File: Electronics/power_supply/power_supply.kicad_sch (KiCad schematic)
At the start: 83 parts, among them IC1 TLV76033DBZR, IC2 LM5069MMX-2_NOPB, J1 Conn_01x02_Male, J10 9801-0-15-15-23-27-10-0, J12 9801-0-15-15-23-27-10-0, J13 9801-0-15-15-23-27-10-0, J14 9801-0-15-15-23-27-10-0, J2 9801-0-15-15-23-27-10-0, J3 Conn_01x02_Male, J4 821-22-002-10-001101, J5 9801-0-15-15-23-27-10-0, J6 Conn_01x04_Male, J7 Conn_01x02_Male, J8 Conn_01x02_Male, J9 Conn_01x02_Pin, Q1 IPD90N04S4L04ATMA1, Q3 BC857, U1 R-78B5.0-2.0, U2 INA226, U3 INA226

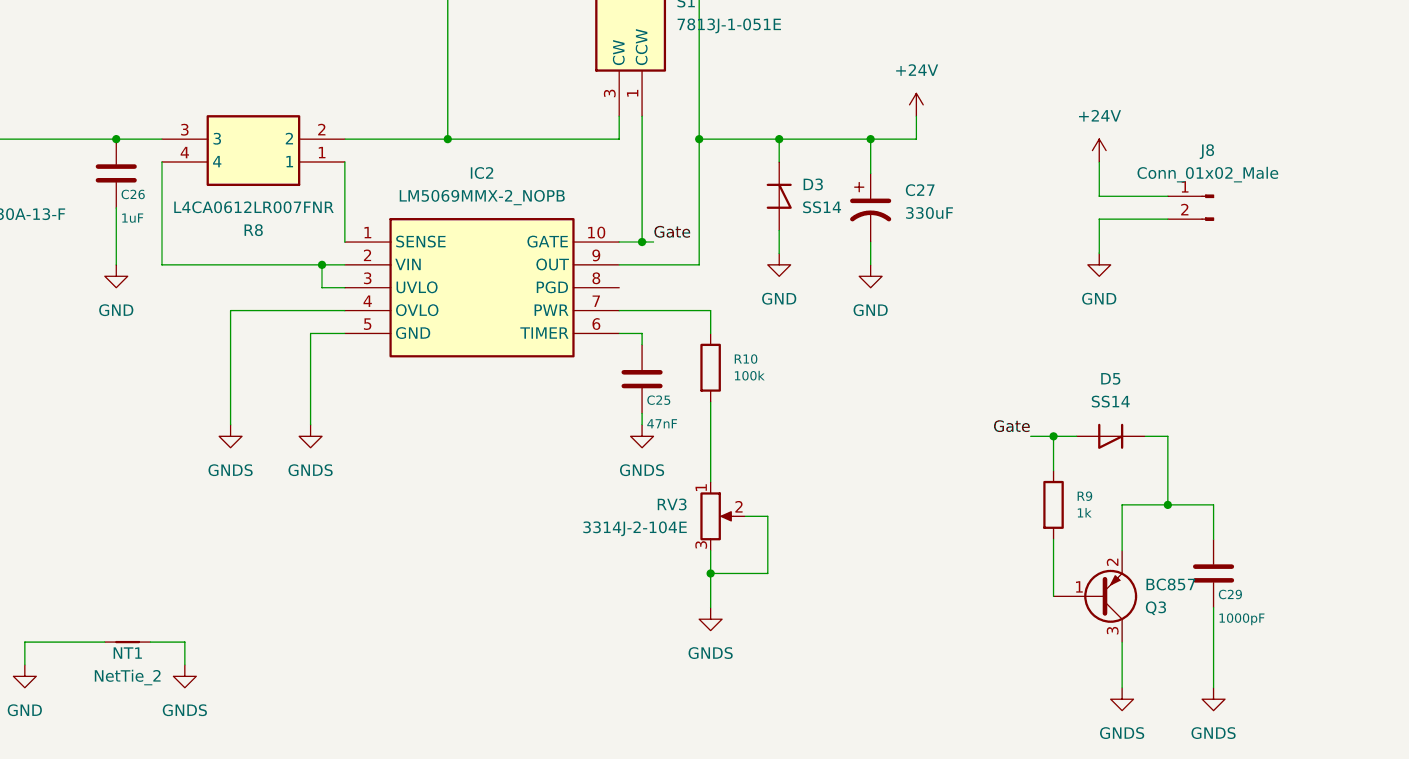
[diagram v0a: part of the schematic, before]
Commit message: PCB fixup
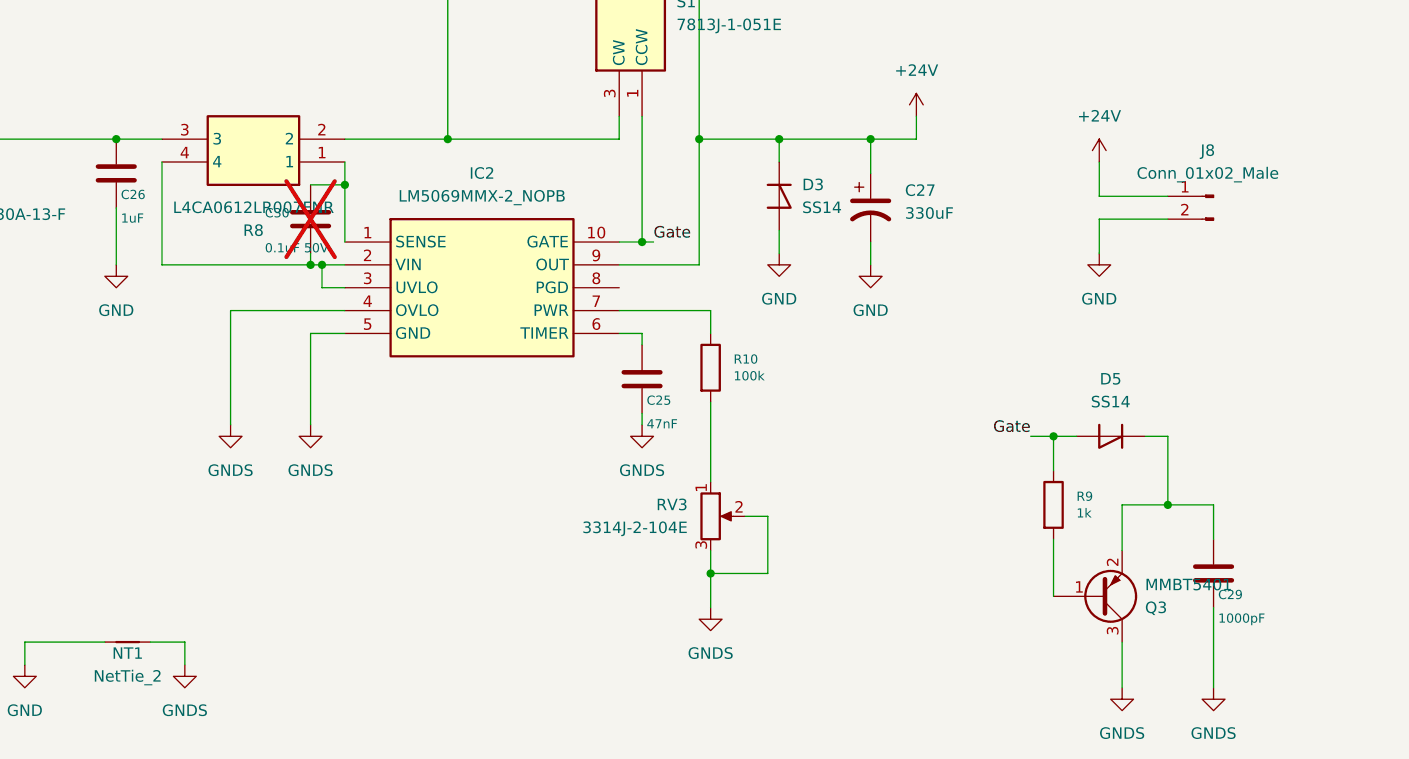
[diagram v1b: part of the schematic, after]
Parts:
- added C30: 0.1uF 50V, Capacitor_SMD:C_0402_1005Metric_Pad0.74x0.62mm_HandSolder, symbol Device:C
- Q3: value BC857 -> MMBT5401; Mouser 583-C857 -> 165-8634
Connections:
- net at IC2.1 (SENSE), R8.1: now also C30.1
- net at IC2.2 (VIN), IC2.3 (UVLO), R8.4: now also C30.2
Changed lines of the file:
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@@
 	)
 	(junction
+		(at 158.75 219.71)
+		(diameter 0)
+		(color 0 0 0 0)
+	)
+	(junction
 		(at 254 246.38)
 		(diameter 0)
@@
 	)
 	(junction
+		(at 162.56 210.82)
+		(diameter 0)
+		(color 0 0 0 0)
+	)
+	(junction
 		(at 351.79 45.72)
 		(diameter 0)
@@
 	(wire
 		(pts
-			(xy 142.24 219.71) (xy 160.02 219.71)
+			(xy 142.24 219.71) (xy 158.75 219.71)
 		)
 		(stroke
@@
 	(wire
 		(pts
-			(xy 162.56 208.28) (xy 162.56 217.17)
+			(xy 162.56 208.28) (xy 162.56 210.82)
 		)
 		(stroke
@@
 	(wire
 		(pts
+			(xy 162.56 210.82) (xy 162.56 217.17)
+		)
+		(stroke
+			(width 0)
+			(type default)
+		)
+	)
+	(wire
+		(pts
 			(xy 341.63 203.2) (xy 346.71 203.2)
 		)
@@
 	(wire
 		(pts
+			(xy 158.75 219.71) (xy 160.02 219.71)
+		)
+		(stroke
+			(width 0)
+			(type default)
+		)
+	)
+	(wire
+		(pts
 			(xy 294.64 95.25) (xy 297.18 95.25)
 		)
@@
 	(wire
 		(pts
+			(xy 158.75 218.44) (xy 158.75 219.71)
+		)
+		(stroke
+			(width 0)
+			(type default)
+		)
+	)
+	(wire
+		(pts
 			(xy 327.66 87.63) (xy 327.66 85.09)
 		)
@@
 	(wire
 		(pts
+			(xy 158.75 210.82) (xy 162.56 210.82)
+		)
+		(stroke
+			(width 0)
+			(type default)
+		)
+	)
+	(wire
+		(pts
 			(xy 74.93 111.76) (xy 74.93 114.3)
 		)
@@
 	(symbol
 		(lib_id "Device:C")
+		(at 158.75 214.63 0)
+		(unit 1)
+		(exclude_from_sim no)
+		(in_bom yes)
+		(on_board yes)
+		(dnp yes)
+		(property "Reference" "C30"
+			(at 153.67 213.36 0)
+			(effects
+				(font
+					(size 1.016 1.016)
+				)
+				(justify left top)
+			)
+		)
+		(property "Value" "0.1uF 50V"
+			(at 153.67 218.44 0)
+			(effects
+				(font
+					(size 1.016 1.016)
+				)
+				(justify left bottom)
+			)
+		)
+		(property "Footprint" "Capacitor_SMD:C_0402_1005Metric_Pad0.74x0.62mm_HandSolder"
+			(at 159.7152 218.44 0)
+			(effects
+				(font
+					(size 1.27 1.27)
+				)
+				(hide yes)
+			)
+		)
+		(property "Datasheet" "~"
+			(at 158.75 214.63 0)
+			(effects
+				(font
+					(size 1.27 1.27)
+				)
+				(hide yes)
+			)
+		)
+		(property "Description" ""
+			(at 158.75 214.63 0)
+			(effects
+				(font
+					(size 1.27 1.27)
+				)
+				(hide yes)
+			)
+		)
+		(property "MF" "TDK"
+			(at 158.75 214.63 0)
+			(effects
+				(font
+					(size 1.27 1.27)
+				)
+				(justify left bottom)
+				(hide yes)
+			)
+		)
+		(property "MPN" "CGA2B3X7R1H104K050BB"
+			(at 158.75 214.63 0)
+			(effects
+				(font
+					(size 1.27 1.27)
+				)
+				(justify left bottom)
+				(hide yes)
+			)
+		)
+		(property "RS" "    247-7824"
+			(at 158.75 214.63 0)
+			(effects
+				(font
+					(size 1.27 1.27)
+				)
+				(hide yes)
+			)
+		)
+		(pin "1"
+		)
+		(pin "2"
+		)
+		(instances
+			(project "power_supply"
+				(path "/700fe2ea-26be-4d6c-908e-561c97acbca5"
+					(reference "C30")
+					(unit 1)
+				)
+			)
+		)
+	)
+	(symbol
+		(lib_id "Device:C")
 		(at 288.29 53.34 0)
 		(unit 1)
@@
 			)
 		)
-		(property "Value" "BC857"
+		(property "Value" "MMBT5401"
 			(at 251.46 255.2701 0)
 			(effects
@@
 			)
 		)
-		(property "Mouser" " 583-C857 "
+		(property "Mouser" "    165-8634"
 			(at 246.38 256.54 0)
 			(effects
